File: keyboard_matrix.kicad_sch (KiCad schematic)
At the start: 308 parts, among them SW2000 MX-LED, SW2001 MX-LED, SW2002 F2, SW2003 F3, SW2004 F4, SW2005 F5, SW2006 F6, SW2007 F7, SW2008 F8, SW2009 F9, SW2010 F10, SW2011 F11, SW2012 F12, SW2013 PrtSc, SW2014 ScrLk, SW2015 Pause, SW2017 1, SW2018 2, SW2019 3, SW2020 4, SW2021 5, SW2022 6, SW2023 7, SW2024 8, SW2025 9, SW2026 0, SW2027 -, SW2028 =, SW2029 Bksp, SW2030 Ins, SW2031 Home, SW2032 PgUp, SW2033 NumLk, SW2034 /, SW2035 *, SW2036 -, SW2037 Tab, SW2038 Q, SW2039 W, SW2040 E, SW2041 R, SW2042 T, SW2043 Y, SW2044 U, SW2045 I, SW2046 O, SW2047 P, SW2048 [, SW2049 ], SW2050 \, SW2051 Del, SW2052 End, SW2053 PgDn, SW2054 7, SW2055 8, SW2056 9, SW2057 +, SW2058 Caps Lock, SW2059 A, SW2060 S, SW2061 D, SW2062 F, SW2063 G, SW2064 H, SW2065 J, SW2066 K, SW2067 L, SW2068 ;, SW2069 ', SW2070 Enter, SW2071 4, SW2072 5, SW2073 6, SW2074 Shift, SW2075 Z, SW2076 X, SW2077 C, SW2078 V, SW2079 B, SW2080 N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

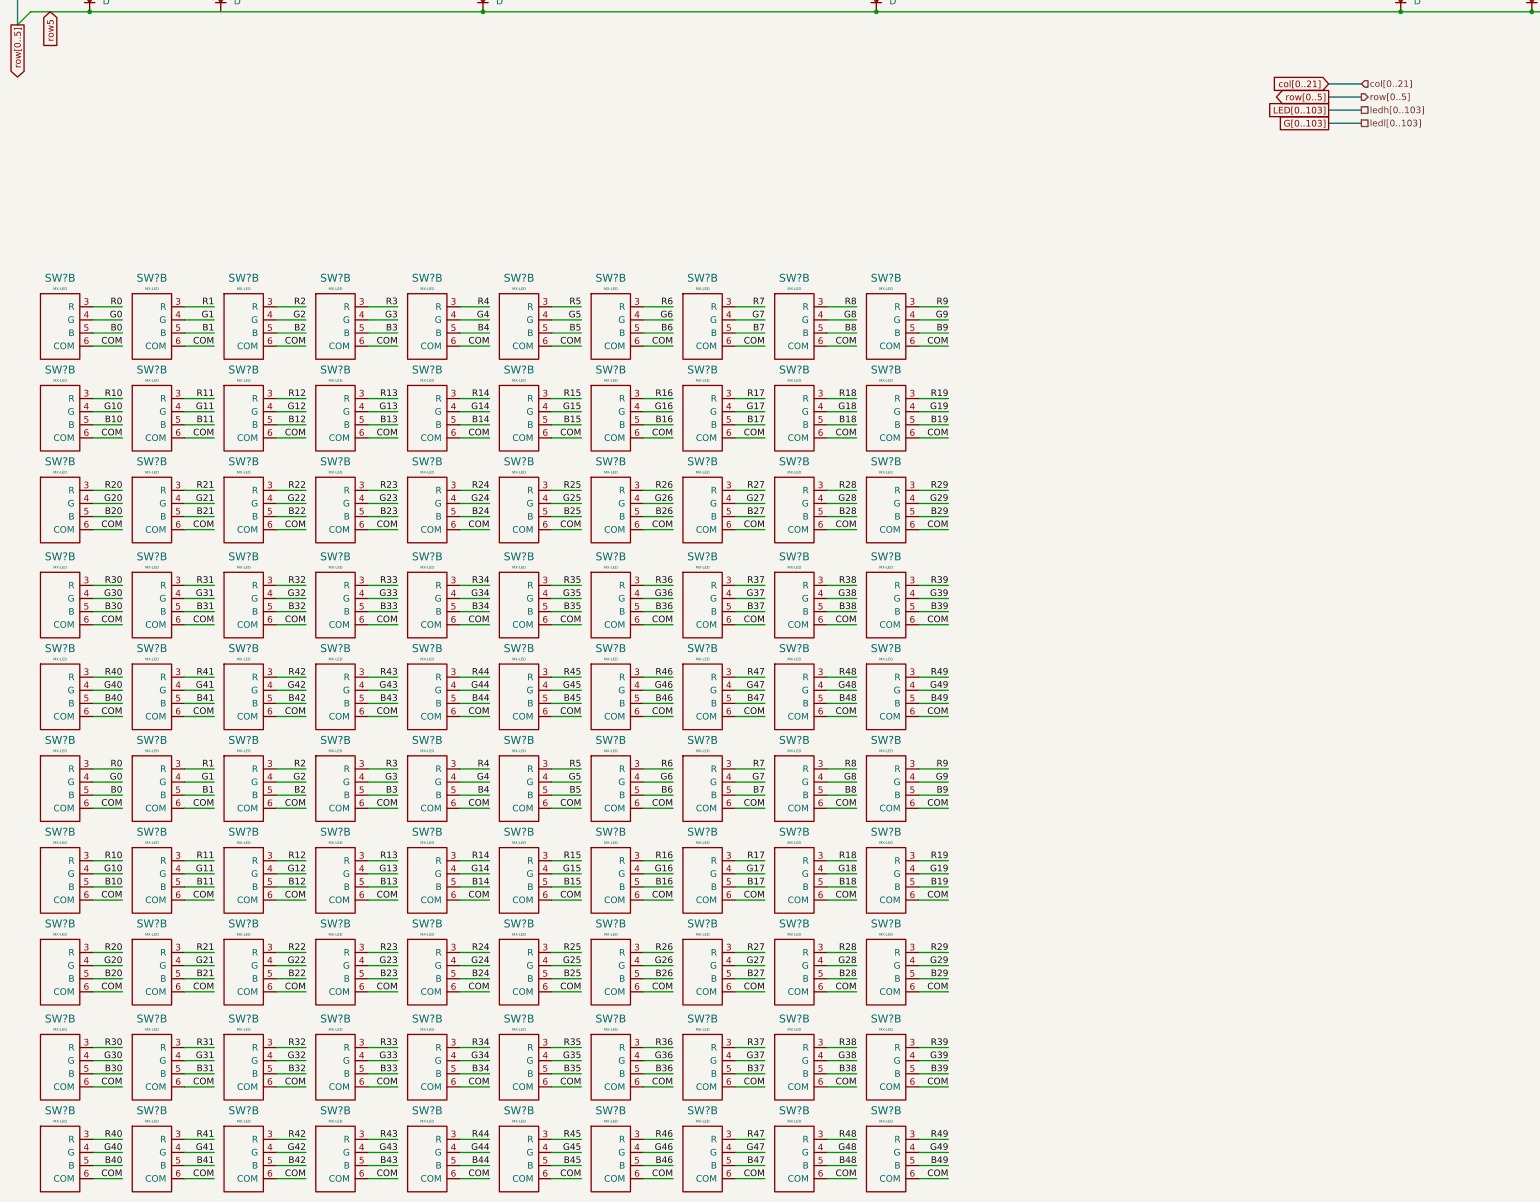
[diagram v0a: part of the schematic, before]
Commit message: fixme
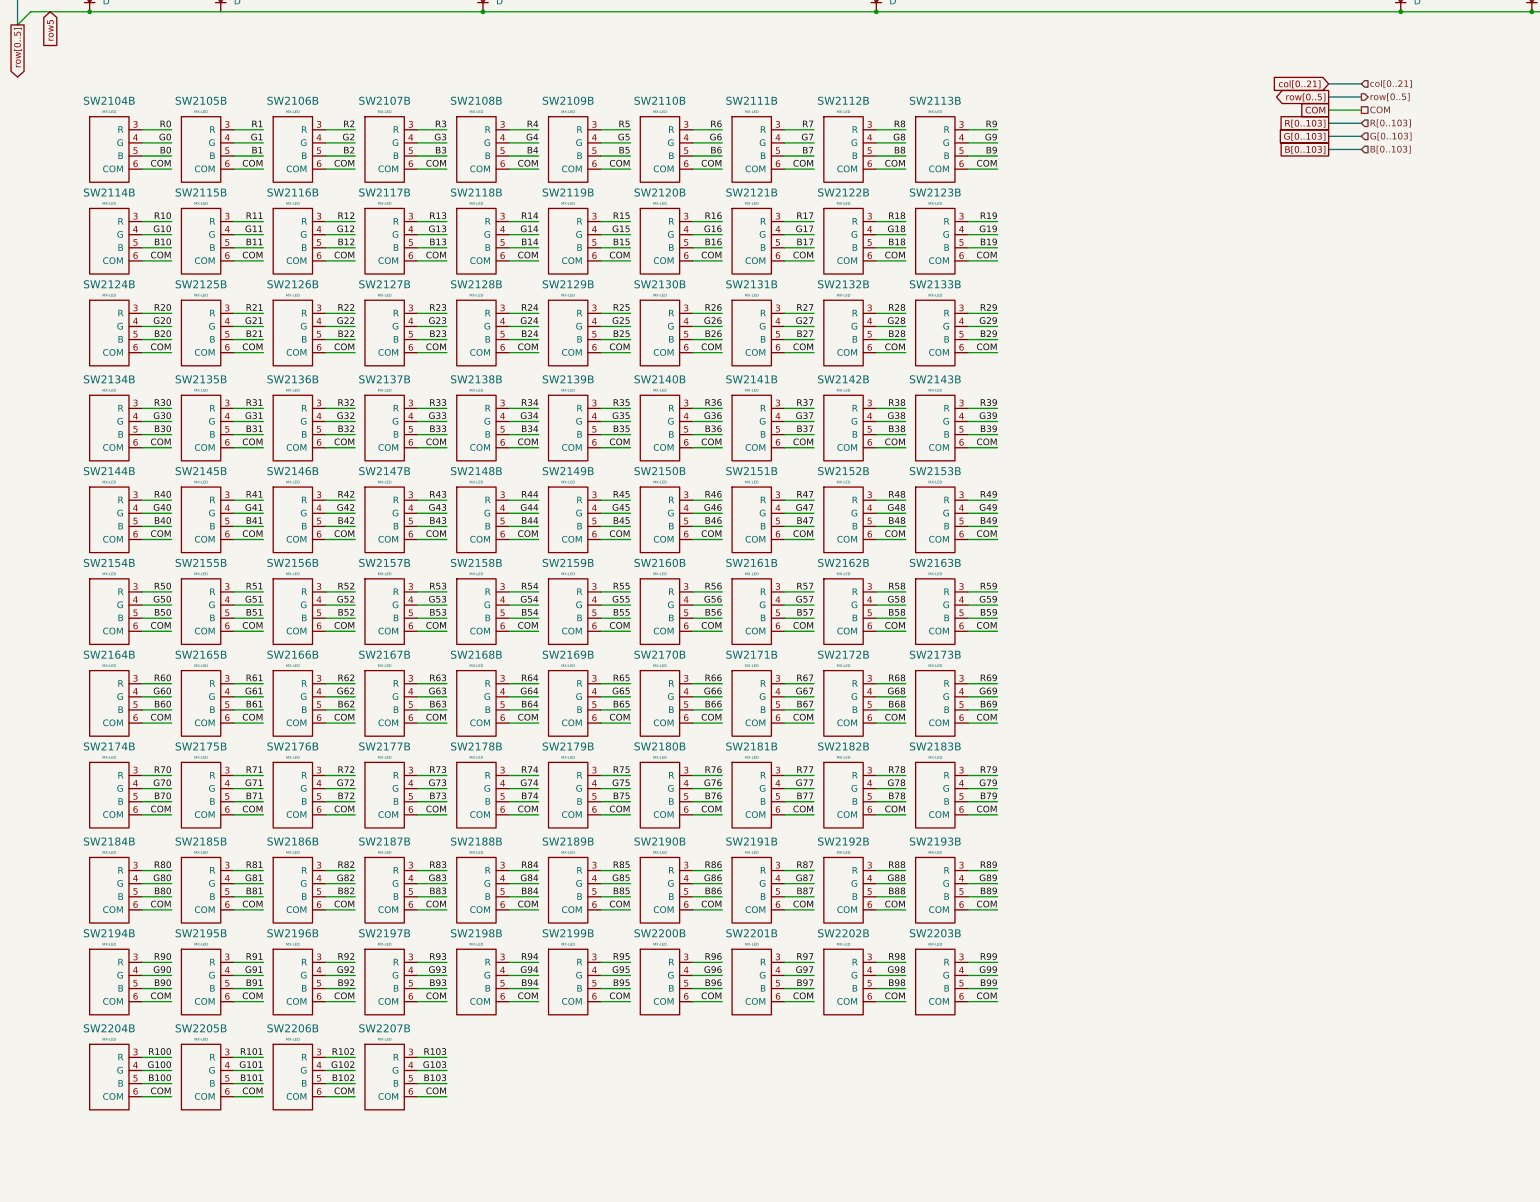
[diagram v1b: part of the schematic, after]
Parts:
- added SW2204, SW2205, SW2206, SW2207: MX-LED, symbol Keyboard:MX-LED
- gave numbers to parts that had none: 100
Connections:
- net B0: no longer SW2154.5 (B)
- net B1: no longer SW2155.5 (B)
- net B10: no longer SW2164.5 (B)
- net B11: no longer SW2165.5 (B)
- net B12: no longer SW2166.5 (B)
- net B13: no longer SW2167.5 (B)
- net B14: no longer SW2168.5 (B)
- net B15: no longer SW2169.5 (B)
- net B16: no longer SW2170.5 (B)
- net B17: no longer SW2171.5 (B)
- net B18: no longer SW2172.5 (B)
- net B19: no longer SW2173.5 (B)
- net B2: no longer SW2156.5 (B)
- net B20: no longer SW2174.5 (B)
- net B21: no longer SW2175.5 (B)
- net B22: no longer SW2176.5 (B)
- net B23: no longer SW2177.5 (B)
- net B24: no longer SW2178.5 (B)
- net B25: no longer SW2179.5 (B)
- net B26: no longer SW2180.5 (B)
- net B27: no longer SW2181.5 (B)
- net B28: no longer SW2182.5 (B)
- net B29: no longer SW2183.5 (B)
- net B3: no longer SW2157.5 (B)
- net B30: no longer SW2184.5 (B)
- net B31: no longer SW2185.5 (B)
- net B32: no longer SW2186.5 (B)
- net B33: no longer SW2187.5 (B)
- net B34: no longer SW2188.5 (B)
- net B35: no longer SW2189.5 (B)
- net B36: no longer SW2190.5 (B)
- net B37: no longer SW2191.5 (B)
- net B38: no longer SW2192.5 (B)
- net B39: no longer SW2193.5 (B)
- net B4: no longer SW2158.5 (B)
- net B40: no longer SW2194.5 (B)
- net B41: no longer SW2195.5 (B)
- net B42: no longer SW2196.5 (B)
- net B43: no longer SW2197.5 (B)
- net B44: no longer SW2198.5 (B)
- net B45: no longer SW2199.5 (B)
- net B46: no longer SW2200.5 (B)
- net B47: no longer SW2201.5 (B)
- net B48: no longer SW2202.5 (B)
- net B49: no longer SW2203.5 (B)
- net B5: no longer SW2159.5 (B)
- net B6: no longer SW2160.5 (B)
- net B7: no longer SW2161.5 (B)
- net B8: no longer SW2162.5 (B)
- net B9: no longer SW2163.5 (B)
- net COM: now also SW2204.6 (COM), SW2205.6 (COM), SW2206.6 (COM), SW2207.6 (COM)
- net G0: no longer SW2154.4 (G)
- net G1: no longer SW2155.4 (G)
- net G10: no longer SW2164.4 (G)
- net G11: no longer SW2165.4 (G)
- net G12: no longer SW2166.4 (G)
- net G13: no longer SW2167.4 (G)
- net G14: no longer SW2168.4 (G)
- net G15: no longer SW2169.4 (G)
- net G16: no longer SW2170.4 (G)
- net G17: no longer SW2171.4 (G)
- net G18: no longer SW2172.4 (G)
- net G19: no longer SW2173.4 (G)
- net G2: no longer SW2156.4 (G)
- net G20: no longer SW2174.4 (G)
- net G21: no longer SW2175.4 (G)
- net G22: no longer SW2176.4 (G)
- net G23: no longer SW2177.4 (G)
- net G24: no longer SW2178.4 (G)
- net G25: no longer SW2179.4 (G)
- net G26: no longer SW2180.4 (G)
- net G27: no longer SW2181.4 (G)
- net G28: no longer SW2182.4 (G)
- net G29: no longer SW2183.4 (G)
- net G3: no longer SW2157.4 (G)
- net G30: no longer SW2184.4 (G)
- net G31: no longer SW2185.4 (G)
- net G32: no longer SW2186.4 (G)
- net G33: no longer SW2187.4 (G)
- net G34: no longer SW2188.4 (G)
- net G35: no longer SW2189.4 (G)
- net G36: no longer SW2190.4 (G)
- net G37: no longer SW2191.4 (G)
- net G38: no longer SW2192.4 (G)
- net G39: no longer SW2193.4 (G)
- net G4: no longer SW2158.4 (G)
- net G40: no longer SW2194.4 (G)
- net G41: no longer SW2195.4 (G)
- net G42: no longer SW2196.4 (G)
- net G43: no longer SW2197.4 (G)
- net G44: no longer SW2198.4 (G)
- net G45: no longer SW2199.4 (G)
- net G46: no longer SW2200.4 (G)
- net G47: no longer SW2201.4 (G)
- net G48: no longer SW2202.4 (G)
- net G49: no longer SW2203.4 (G)
- net G5: no longer SW2159.4 (G)
- net G6: no longer SW2160.4 (G)
- net G7: no longer SW2161.4 (G)
- net G8: no longer SW2162.4 (G)
- net G9: no longer SW2163.4 (G)
- net R0: no longer SW2154.3 (R)
- net R1: no longer SW2155.3 (R)
- net R10: no longer SW2164.3 (R)
- net R11: no longer SW2165.3 (R)
- net R12: no longer SW2166.3 (R)
- net R13: no longer SW2167.3 (R)
- net R14: no longer SW2168.3 (R)
- net R15: no longer SW2169.3 (R)
- net R16: no longer SW2170.3 (R)
- net R17: no longer SW2171.3 (R)
- net R18: no longer SW2172.3 (R)
- net R19: no longer SW2173.3 (R)
- net R2: no longer SW2156.3 (R)
- net R20: no longer SW2174.3 (R)
- net R21: no longer SW2175.3 (R)
- net R22: no longer SW2176.3 (R)
- net R23: no longer SW2177.3 (R)
- net R24: no longer SW2178.3 (R)
- net R25: no longer SW2179.3 (R)
- net R26: no longer SW2180.3 (R)
- net R27: no longer SW2181.3 (R)
- net R28: no longer SW2182.3 (R)
- net R29: no longer SW2183.3 (R)
- net R3: no longer SW2157.3 (R)
- net R30: no longer SW2184.3 (R)
- net R31: no longer SW2185.3 (R)
- net R32: no longer SW2186.3 (R)
- net R33: no longer SW2187.3 (R)
- net R34: no longer SW2188.3 (R)
- net R35: no longer SW2189.3 (R)
- net R36: no longer SW2190.3 (R)
- net R37: no longer SW2191.3 (R)
- net R38: no longer SW2192.3 (R)
- net R39: no longer SW2193.3 (R)
- net R4: no longer SW2158.3 (R)
- net R40: no longer SW2194.3 (R)
- net R41: no longer SW2195.3 (R)
- net R42: no longer SW2196.3 (R)
- net R43: no longer SW2197.3 (R)
- net R44: no longer SW2198.3 (R)
- net R45: no longer SW2199.3 (R)
- net R46: no longer SW2200.3 (R)
- net R47: no longer SW2201.3 (R)
- net R48: no longer SW2202.3 (R)
- net R49: no longer SW2203.3 (R)
- net R5: no longer SW2159.3 (R)
- net R6: no longer SW2160.3 (R)
- net R7: no longer SW2161.3 (R)
- net R8: no longer SW2162.3 (R)
- net R9: no longer SW2163.3 (R)
- new net B100: SW2204.5 (B)
- new net B101: SW2205.5 (B)
- new net B102: SW2206.5 (B)
- new net B103: SW2207.5 (B)
- new net B50: SW2154.5 (B)
- new net B51: SW2155.5 (B)
- new net B52: SW2156.5 (B)
- new net B53: SW2157.5 (B)
- new net B54: SW2158.5 (B)
- new net B55: SW2159.5 (B)
- new net B56: SW2160.5 (B)
- new net B57: SW2161.5 (B)
- new net B58: SW2162.5 (B)
- new net B59: SW2163.5 (B)
- new net B60: SW2164.5 (B)
- new net B61: SW2165.5 (B)
- new net B62: SW2166.5 (B)
- new net B63: SW2167.5 (B)
- new net B64: SW2168.5 (B)
- new net B65: SW2169.5 (B)
- new net B66: SW2170.5 (B)
- new net B67: SW2171.5 (B)
- new net B68: SW2172.5 (B)
- new net B69: SW2173.5 (B)
- new net B70: SW2174.5 (B)
- new net B71: SW2175.5 (B)
- new net B72: SW2176.5 (B)
- new net B73: SW2177.5 (B)
- new net B74: SW2178.5 (B)
- new net B75: SW2179.5 (B)
- new net B76: SW2180.5 (B)
- new net B77: SW2181.5 (B)
- new net B78: SW2182.5 (B)
- new net B79: SW2183.5 (B)
- new net B80: SW2184.5 (B)
- new net B81: SW2185.5 (B)
- new net B82: SW2186.5 (B)
- new net B83: SW2187.5 (B)
- new net B84: SW2188.5 (B)
- new net B85: SW2189.5 (B)
- new net B86: SW2190.5 (B)
- new net B87: SW2191.5 (B)
- new net B88: SW2192.5 (B)
- new net B89: SW2193.5 (B)
- new net B90: SW2194.5 (B)
- new net B91: SW2195.5 (B)
- new net B92: SW2196.5 (B)
- new net B93: SW2197.5 (B)
- new net B94: SW2198.5 (B)
- new net B95: SW2199.5 (B)
- new net B96: SW2200.5 (B)
- new net B97: SW2201.5 (B)
- new net B98: SW2202.5 (B)
- new net B99: SW2203.5 (B)
- new net G100: SW2204.4 (G)
- new net G101: SW2205.4 (G)
- new net G102: SW2206.4 (G)
- new net G103: SW2207.4 (G)
- new net G50: SW2154.4 (G)
- new net G51: SW2155.4 (G)
- new net G52: SW2156.4 (G)
- new net G53: SW2157.4 (G)
- new net G54: SW2158.4 (G)
- new net G55: SW2159.4 (G)
- new net G56: SW2160.4 (G)
- new net G57: SW2161.4 (G)
- new net G58: SW2162.4 (G)
- new net G59: SW2163.4 (G)
- new net G60: SW2164.4 (G)
- new net G61: SW2165.4 (G)
- new net G62: SW2166.4 (G)
- new net G63: SW2167.4 (G)
- new net G64: SW2168.4 (G)
- new net G65: SW2169.4 (G)
- new net G66: SW2170.4 (G)
- new net G67: SW2171.4 (G)
- new net G68: SW2172.4 (G)
- new net G69: SW2173.4 (G)
- new net G70: SW2174.4 (G)
- new net G71: SW2175.4 (G)
- new net G72: SW2176.4 (G)
- new net G73: SW2177.4 (G)
- new net G74: SW2178.4 (G)
- new net G75: SW2179.4 (G)
- new net G76: SW2180.4 (G)
- new net G77: SW2181.4 (G)
- new net G78: SW2182.4 (G)
- new net G79: SW2183.4 (G)
- new net G80: SW2184.4 (G)
- new net G81: SW2185.4 (G)
- new net G82: SW2186.4 (G)
- new net G83: SW2187.4 (G)
- new net G84: SW2188.4 (G)
- new net G85: SW2189.4 (G)
- new net G86: SW2190.4 (G)
- new net G87: SW2191.4 (G)
- new net G88: SW2192.4 (G)
- new net G89: SW2193.4 (G)
- new net G90: SW2194.4 (G)
- new net G91: SW2195.4 (G)
- new net G92: SW2196.4 (G)
- new net G93: SW2197.4 (G)
- new net G94: SW2198.4 (G)
- new net G95: SW2199.4 (G)
- new net G96: SW2200.4 (G)
- new net G97: SW2201.4 (G)
- new net G98: SW2202.4 (G)
- new net G99: SW2203.4 (G)
- new net R100: SW2204.3 (R)
- new net R101: SW2205.3 (R)
- new net R102: SW2206.3 (R)
- new net R103: SW2207.3 (R)
- new net R50: SW2154.3 (R)
- new net R51: SW2155.3 (R)
- new net R52: SW2156.3 (R)
- new net R53: SW2157.3 (R)
- new net R54: SW2158.3 (R)
- new net R55: SW2159.3 (R)
- new net R56: SW2160.3 (R)
- new net R57: SW2161.3 (R)
- new net R58: SW2162.3 (R)
- new net R59: SW2163.3 (R)
- new net R60: SW2164.3 (R)
- new net R61: SW2165.3 (R)
- new net R62: SW2166.3 (R)
- new net R63: SW2167.3 (R)
- new net R64: SW2168.3 (R)
- new net R65: SW2169.3 (R)
- new net R66: SW2170.3 (R)
- new net R67: SW2171.3 (R)
- new net R68: SW2172.3 (R)
- new net R69: SW2173.3 (R)
- new net R70: SW2174.3 (R)
- new net R71: SW2175.3 (R)
- new net R72: SW2176.3 (R)
- new net R73: SW2177.3 (R)
- new net R74: SW2178.3 (R)
- new net R75: SW2179.3 (R)
- new net R76: SW2180.3 (R)
- new net R77: SW2181.3 (R)
- new net R78: SW2182.3 (R)
- new net R79: SW2183.3 (R)
- new net R80: SW2184.3 (R)
- new net R81: SW2185.3 (R)
- new net R82: SW2186.3 (R)
- new net R83: SW2187.3 (R)
- new net R84: SW2188.3 (R)
- new net R85: SW2189.3 (R)
- new net R86: SW2190.3 (R)
- new net R87: SW2191.3 (R)
- new net R88: SW2192.3 (R)
- new net R89: SW2193.3 (R)
- new net R90: SW2194.3 (R)
- new net R91: SW2195.3 (R)
- new net R92: SW2196.3 (R)
- new net R93: SW2197.3 (R)
- new net R94: SW2198.3 (R)
- new net R95: SW2199.3 (R)
- new net R96: SW2200.3 (R)
- new net R97: SW2201.3 (R)
- new net R98: SW2202.3 (R)
- new net R99: SW2203.3 (R)
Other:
- moved on the sheet: SW2104B, SW2105B, SW2106B, SW2107B, SW2108B, SW2109B, SW2110B, SW2111B, SW2112B, SW2113B, SW2114B, SW2115B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
